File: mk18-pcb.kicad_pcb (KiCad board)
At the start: 2 copper layers, 121.5 x 66 mm, 48 parts

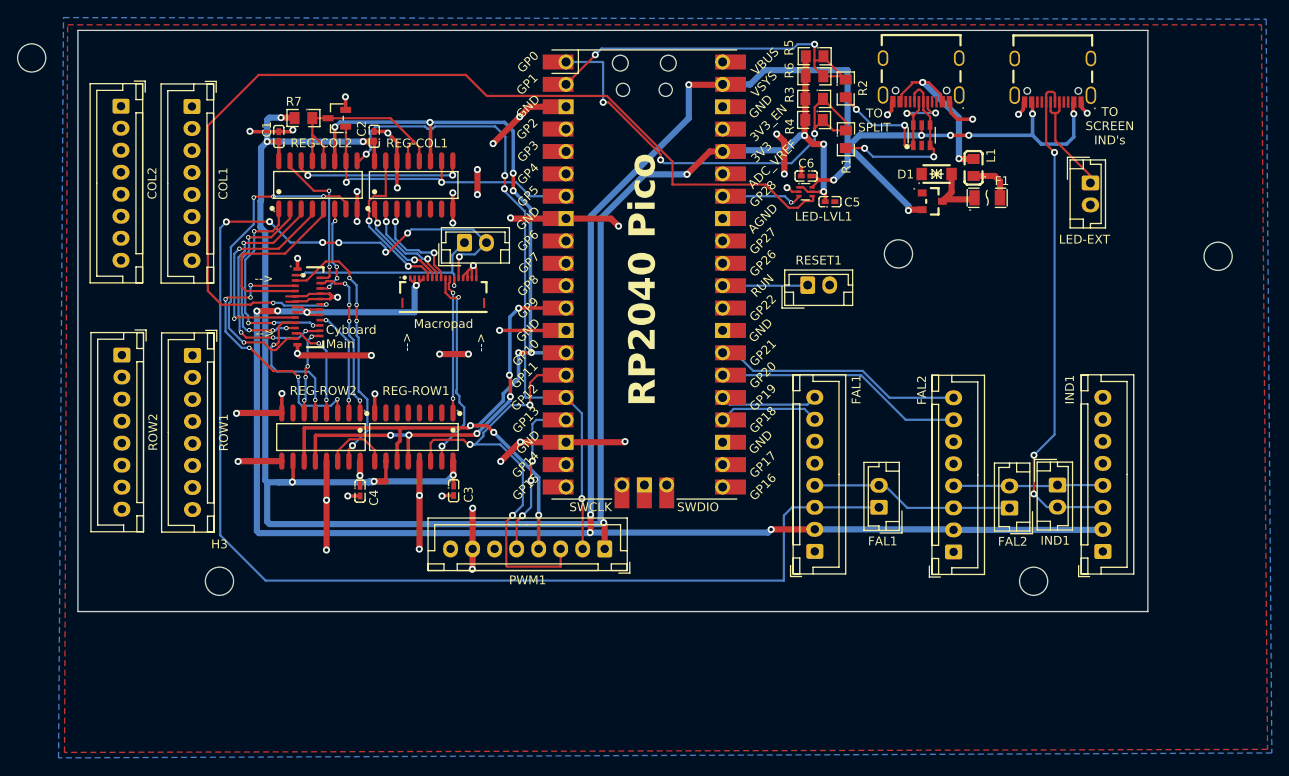
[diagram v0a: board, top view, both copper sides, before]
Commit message: jan4 updates
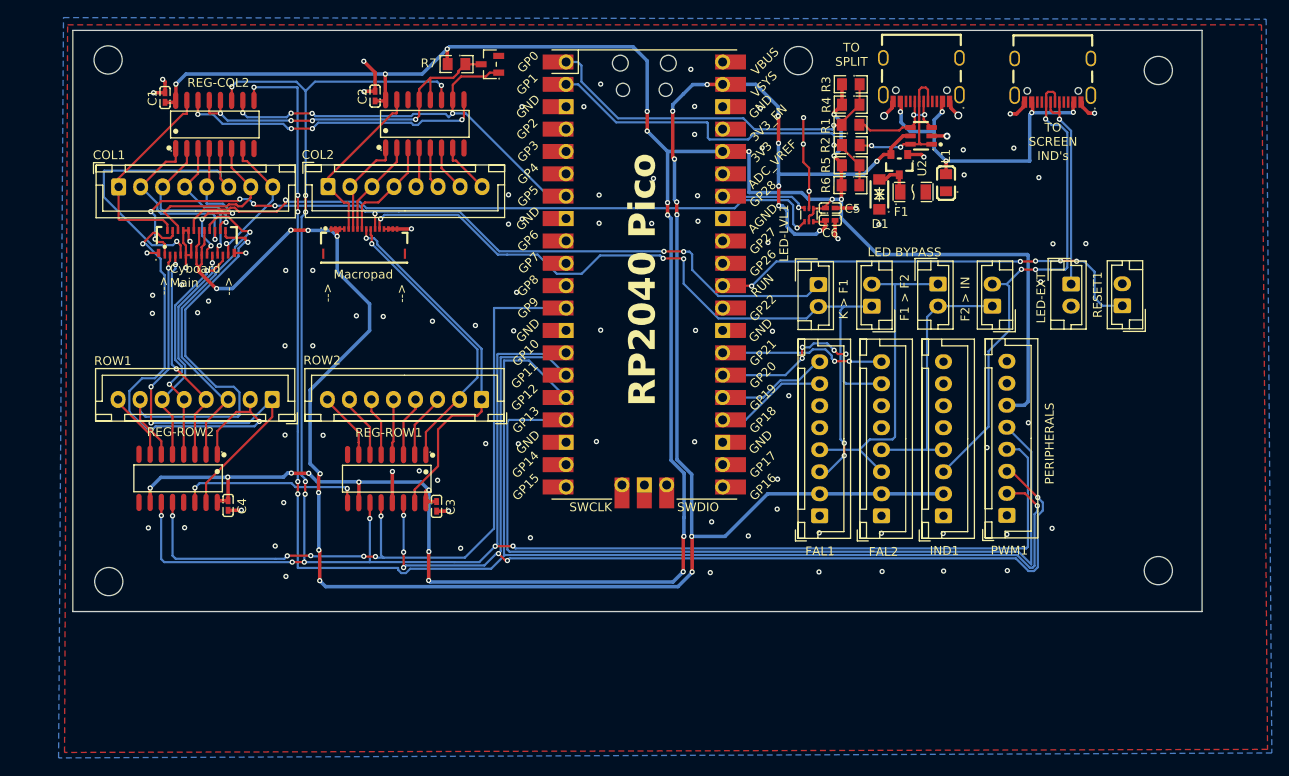
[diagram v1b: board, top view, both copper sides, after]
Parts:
- removed BOOST-CONVERT1: SRV0504, ct-kicad:SOT-23-6_L2.9-W1.6-P0.95-LS2.8-BL
- added U2: AZC199-04S-MS, ct-kicad:TSOT-23-6_L2.9-W1.6-P0.95-LS2.8-BL, F.Cu at (191.4, 82.7)
- moved H2 52.6 mm to (177.5, 74.1)
- moved PWM1 45.8 mm to (201.2, 125.8), turned to 90 degrees
- moved ROW2 41.1 mm to (141.5, 112.6), turned to 180 degrees
- moved LED-MACRO1 40.5 mm to (179.8, 99.6), turned to -90 degrees
- moved H5 36.1 mm to (218.4, 75.3)
- moved RESET1 35.8 mm to (214.3, 102.0), turned to 90 degrees
- moved LED-FAL2 26.7 mm to (193.4, 99.5), turned to -90 degrees
- moved COL2 25.2 mm to (124.1, 88.5), turned to 0 degrees
- moved LED-FAL1 22.9 mm to (185.9, 102.0)
- moved LED-IND1 21.6 mm to (199.5, 102.0), turned to 90 degrees
- moved IND1 18.5 mm to (194.0, 125.8)
- moved R7 18.4 mm to (138.7, 74.5)
- moved COL_CS_MOS1 18.4 mm to (142.5, 74.6)
- moved REG-ROW2 16.9 mm to (107.1, 121.6)
- moved C4 15.1 mm to (112.8, 124.7)
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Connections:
- PWM1 pad 1: +3V3 -> GND
- PWM1 pad 6: unconnected-(PWM1-Pin_6-Pad6) -> +3V3
- PWM1 pad 7: GND -> unconnected-(PWM1-Pin_7-Pad7)
- SCREEN1 pad A4: VCC -> Serial_VBUS
- SCREEN1 pad A9: VCC -> Serial_VBUS
- SCREEN1 pad B4: VCC -> Serial_VBUS
- SCREEN1 pad B9: VCC -> Serial_VBUS
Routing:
- net SPI1_CLK: track 116.7 -> 237.5 mm, vias 9 -> 12
- net SPI1_MISO: track 73.6 -> 188.5 mm, vias 4 -> 6
- net GND: track 163.2 -> 56.3 mm, vias 45 -> 99
- net PMW_CS: track 18.9 -> 98.2 mm, vias 3 -> 0
- net SPI1_MOSI: track 50.0 -> 125.0 mm, vias 3 -> 6
- net LED_FAL1_DI: track 159.7 -> 86.8 mm, vias 7 -> 5
- net +3V3: track 228.0 -> 296.8 mm, vias 12 -> 22
- net LED_KEYS_DO: track 24.3 -> 90.4 mm, vias 2 -> 8
- net reset: track 9.68 -> 50.4 mm, vias 0 -> 5
- net row6: track 9.99 -> 50.3 mm, vias 4 -> 1
- net LED_KEYS_DI: track 113.8 -> 75.7 mm
- net ROW_CS: track 46.2 -> 83.9 mm
- net row1: track 18.5 -> 53.8 mm, vias 4 -> 2
- net VCC: track 291.9 -> 256.8 mm, vias 15 -> 21
- net row2: track 12.4 -> 38.2 mm, vias 2 -> 1
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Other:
- board size 121.5 x 66 mm -> 128.2 x 66 mm
- board text added: "F1 > F2"
- board text added: "F2 > IN"
- board text added: "K > F1"
- board text added: "LED BYPASS"
- board text added: "PERIPHERALS"
